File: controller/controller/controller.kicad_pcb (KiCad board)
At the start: 2 copper layers, 97.3 x 120.4 mm, 52 parts, among them J1-I1 SJ-3524-SMT, J11-O1 SJ-3524-SMT, SW1 SW_Omron_B3FS, U1 H11L1, U2 74HC4051, U3 Pico, U4 I2S_PCM_51XX_SOUNDCARD

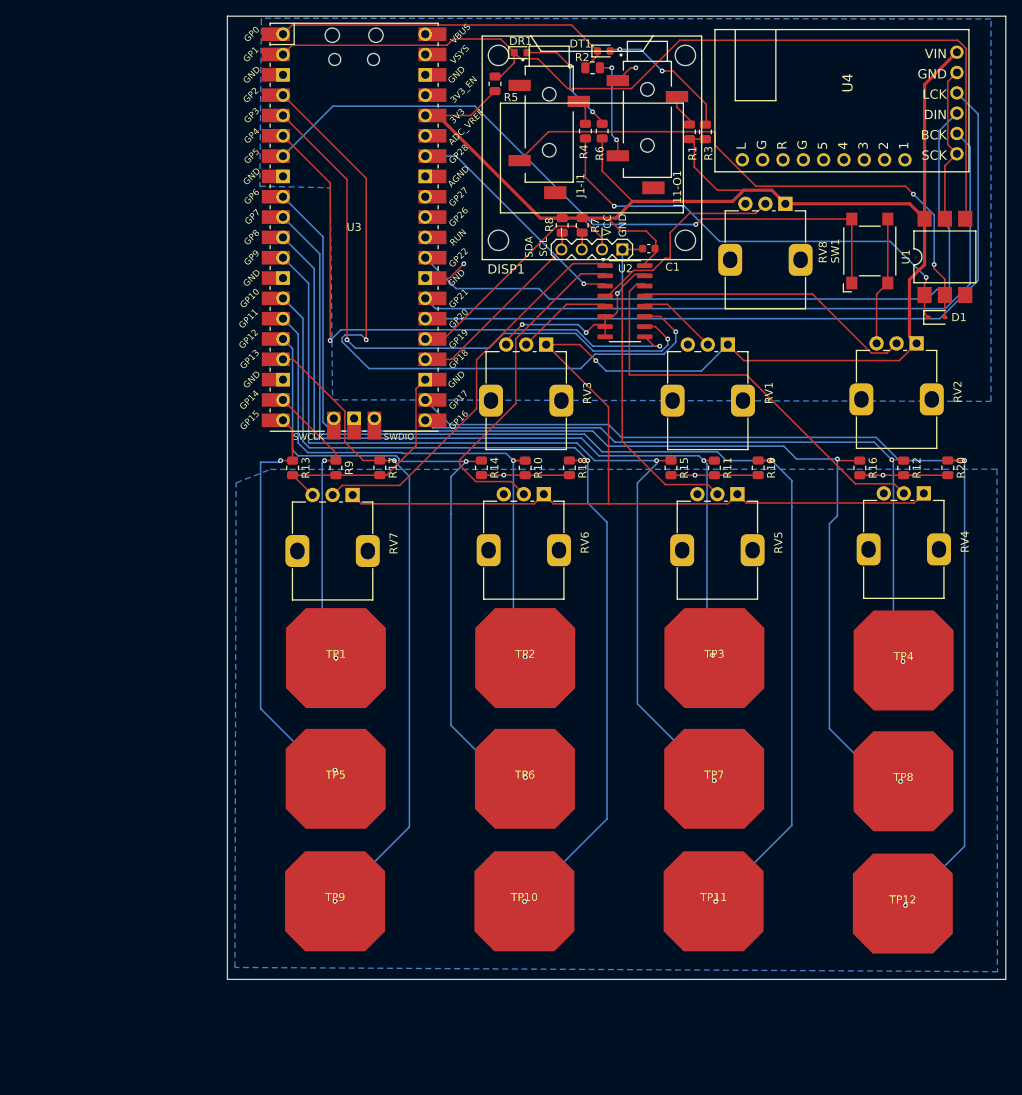
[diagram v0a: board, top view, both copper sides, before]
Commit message: prototype v2
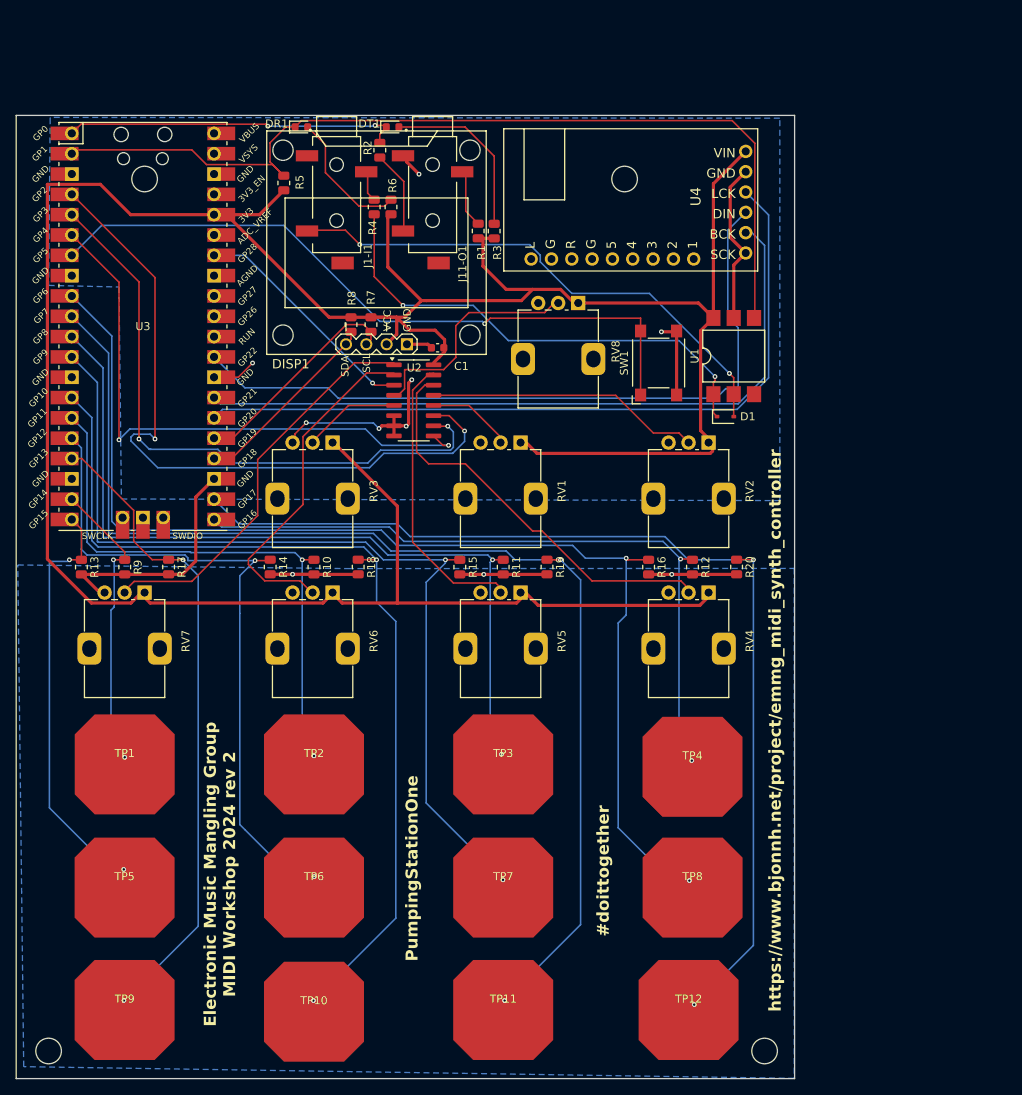
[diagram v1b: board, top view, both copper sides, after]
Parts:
- added Hole1: MountingHole_3.2mm_M3, MountingHole:MountingHole_3.2mm_M3, F.Cu at (53.6, 41.2)
- added Hole2: MountingHole_3.2mm_M3, MountingHole:MountingHole_3.2mm_M3, F.Cu at (113.6, 41.2)
- added Hole3: MountingHole_3.2mm_M3, MountingHole:MountingHole_3.2mm_M3, F.Cu at (41.6, 150.2)
- added Hole4: MountingHoles are 3.2mm_M3, MountingHole:MountingHole_3.2mm_M3, F.Cu at (131.1, 150.2)
- moved SW1 29.9 mm to (117.8, 64.2)
- moved RV5 29.8 mm to (100.6, 92.9)
- moved RV4 29.6 mm to (124.1, 92.9)
- moved TP12 29.5 mm to (121.6, 144.2)
- moved DISP1 29.4 mm to (82.6, 49.2)
- moved RV3 29.4 mm to (77.1, 74.2)
- moved TP10 29.3 mm to (74.8, 144.4)
- moved TP5 29.3 mm to (51.1, 128.9)
- moved TP6 29.3 mm to (74.8, 128.9)
- moved TP7 29.3 mm to (98.4, 128.9)
- moved TP9 29.2 mm to (51.1, 144.2)
- moved TP11 29.2 mm to (98.4, 144.2)
- moved C1 29.2 mm to (90.2, 62.3)
- moved R1 29.2 mm to (95.3, 47.7)
- moved R10 29.2 mm to (74.8, 89.7)
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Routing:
- net +3V3: track 309.3 -> 370.0 mm, vias 1 -> 0
- net GND: track 136.2 -> 129.8 mm, vias 8 -> 10
- net Net-(D1-A): track 71.9 -> 66.1 mm
- net unconnected-(R3-Pad2): track 17.6 -> 21.9 mm, vias 2 -> 0
- net unconnected-(D1-K-Pad1): track 57.9 -> 60.8 mm
- net unconnected-(J11-O1-Pad3): track 4.38 -> 7.13 mm
- net unconnected-(J11-O1-Pad2): track 12.8 -> 10.4 mm, vias 2 -> 0
- net unconnected-(DR1-A-Pad2): track 15.0 -> 16.9 mm, vias 2 -> 0
- net /POT8: track 26.7 -> 28.5 mm
- net /POT4: track 53.2 -> 51.6 mm
- net /Midi Output 1/TX: track 43.9 -> 42.3 mm, vias 0 -> 2
- net /POT1: track 9.97 -> 11.0 mm
- net unconnected-(J1-I1-Pad3): track 3.14 -> 3.93 mm
- net /POT2: track 35.0 -> 34.3 mm
- net /SDA: track 24.8 -> 24.2 mm
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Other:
- board text added: "#doittogether"
- board text added: "AUDIO OUT"
- board text added: "Electronic Music Mangling Group MIDI Workshop 2024 rev 2"
- board text added: "MIDI IN"
- board text added: "MIDI OUT"
- board text added: "PumpingStationOne"
- board text added: "USB"
- board text added: "Warning, the edge cuts are not precise, always favor internal dimensions."
- board text added: "https://www.bjonnh.net/project/emmg_midi_synth_controller"
